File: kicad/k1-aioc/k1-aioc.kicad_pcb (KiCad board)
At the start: 2 copper layers, 21 x 31.5 mm, 40 parts, among them J1 12401832E402A, J2 Conn_01x07_Male, Q1 BC847BS, U1 LP2985-3.3, U2 STM32F373CBTx, Y1 8MHz/20pF

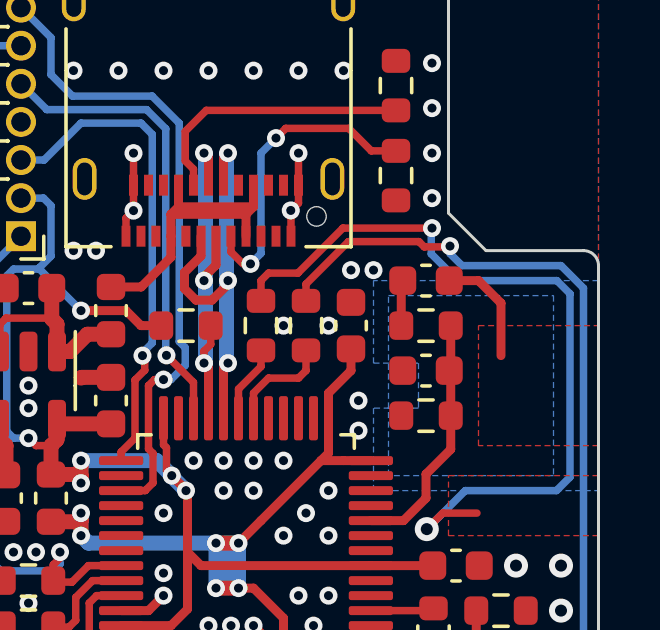
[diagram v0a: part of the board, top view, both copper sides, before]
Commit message: Added missing biasing resistor on AFIN
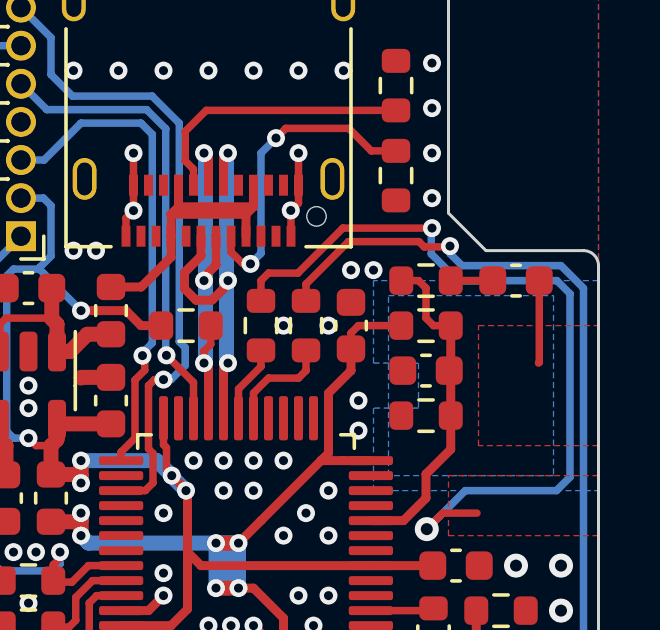
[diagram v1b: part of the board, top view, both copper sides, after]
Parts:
- added R16: 5.1K, Resistor_SMD:R_0603_1608Metric, F.Cu at (118.8, 92.0)
- R3: value 2.2K -> 5.1K
- moved C14 3.00 mm to (121.8, 90.5)
- moved R5 1.50 mm to (118.8, 90.5), turned to 0 degrees
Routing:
- net /AFIN: track 8.24 -> 11.1 mm
- net +3.3VA: track 29.2 -> 31.5 mm
- net /RADIO-SPK: track 3.79 -> 2.76 mm
